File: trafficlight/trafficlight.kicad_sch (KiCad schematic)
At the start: 7 parts, among them J1 Power, U1 LM555xM, U2 4017

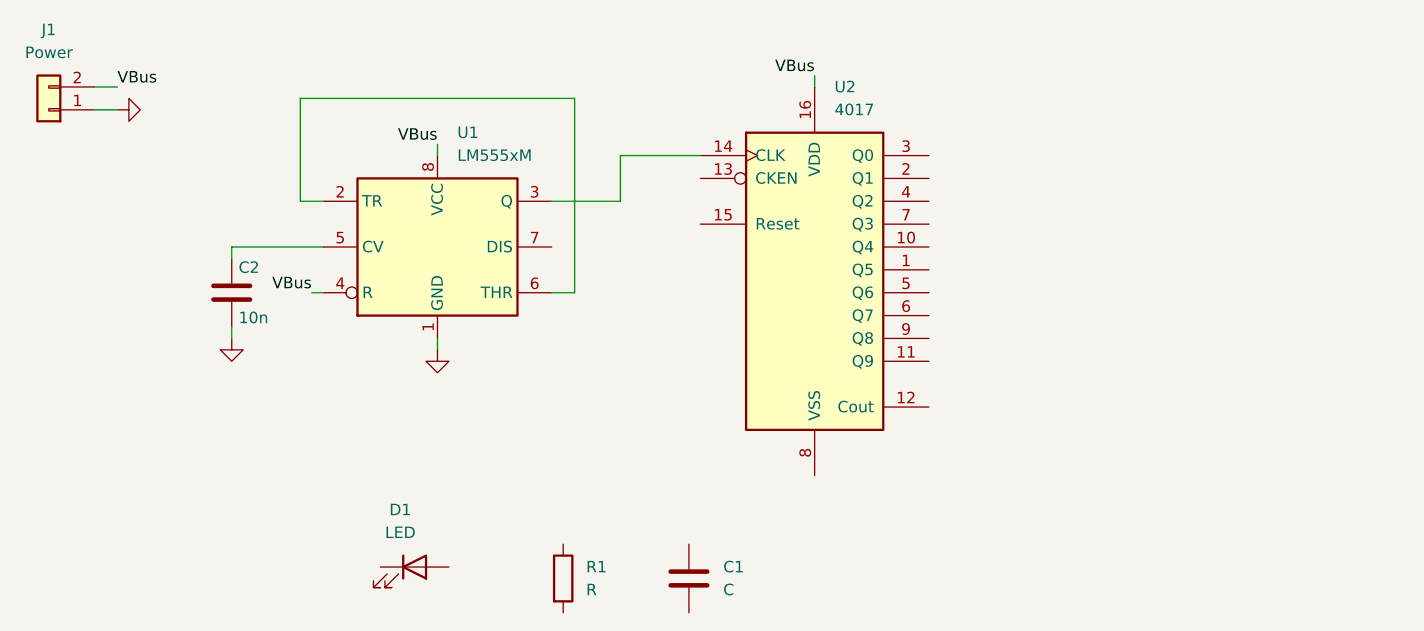
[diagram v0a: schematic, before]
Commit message: Update PCB
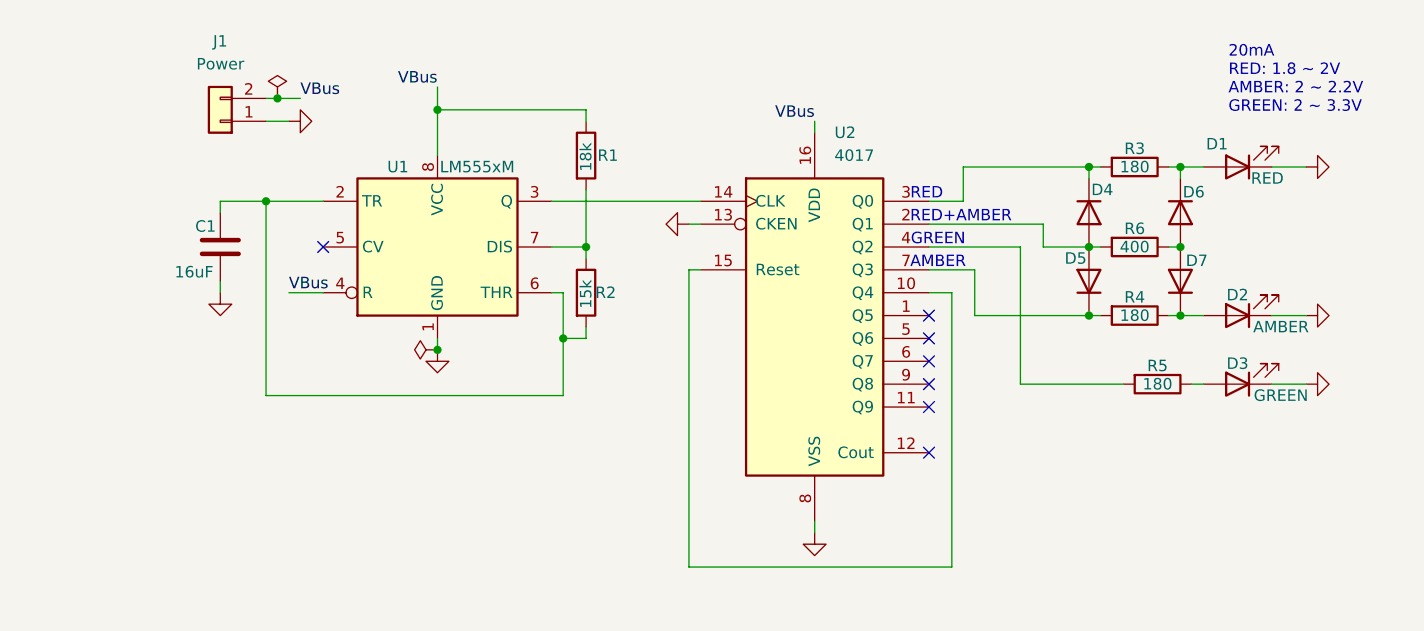
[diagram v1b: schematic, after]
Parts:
- removed C1: C, symbol Device:C
- added D2: AMBER, LED_THT:LED_D4.0mm, symbol Device:LED
- added D3: GREEN, LED_THT:LED_D4.0mm, symbol Device:LED
- added D4, D5, D6, D7: D, Diode_SMD:D_0603_1608Metric_Pad1.05x0.95mm_HandSolder, symbol Device:D
- added R1: 18k, Resistor_SMD:R_0603_1608Metric_Pad0.98x0.95mm_HandSolder, symbol Device:R
- added R2: 15k, Resistor_SMD:R_0603_1608Metric_Pad0.98x0.95mm_HandSolder, symbol Device:R
- added R4, R5: 180, Resistor_SMD:R_0603_1608Metric_Pad0.98x0.95mm_HandSolder, symbol Device:R
- added R6: 400, Resistor_SMD:R_0603_1608Metric_Pad0.98x0.95mm_HandSolder, symbol Device:R
- C1: renamed from C2; value 10n -> 16uF; footprint (none) -> Capacitor_SMD:C_0603_1608Metric_Pad1.08x0.95mm_HandSolder
- D1: value LED -> RED; footprint (none) -> LED_THT:LED_D4.0mm
- J1: footprint (none) -> Connector_PinHeader_2.54mm:PinHeader_1x02_P2.54mm_Vertical
- R3: renamed from R1; value R -> 180; footprint (none) -> Resistor_SMD:R_0603_1608Metric_Pad0.98x0.95mm_HandSolder
- U2: footprint (none) -> Package_DIP:DIP-16_W7.62mm
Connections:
- net GND: now also D1.1 (K), U2.13 (CKEN), U2.8 (VSS), D2.1 (K), D3.1 (K)
- net VBus: now also R1.1
- net at U1.2 (TR), U1.6 (THR): now also C1.1, R2.2
- net at U1.5 (CV): no longer C1.1
- net at U1.7 (DIS): now also R1.2, R2.1
- net at R3.1: now also D1.2 (A), D6.1 (K)
- net at R3.2: now also U2.3 (Q0), D4.1 (K)
- net at U2.10 (Q4): now also U2.15 (Reset)
- net at U2.2 (Q1): now also D4.2 (A), D5.2 (A), R6.2
- net at U2.4 (Q2): now also R5.2
- net at U2.7 (Q3): now also D5.1 (K), R4.2
- new net: D3.2 (A), R5.1
- new net: D2.2 (A), D7.1 (K), R4.1
- new net: D6.2 (A), D7.2 (A), R6.1
- no-connect marks 0 -> 7
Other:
- note added: "20mA RED: 1.8 ~ 2V AMBER: 2 ~ 2.2V GREEN: 2 ~ 3.3V"
- note added: "AMBER"
- note added: "GREEN"
- note added: "RED"
- note added: "RED+AMBER"
- moved on the sheet: C1, D1, J1, R3, U2
